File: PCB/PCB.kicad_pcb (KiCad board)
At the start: 2 copper layers, 17 parts, among them U1 ESP32-WROOM-32E-N8R2

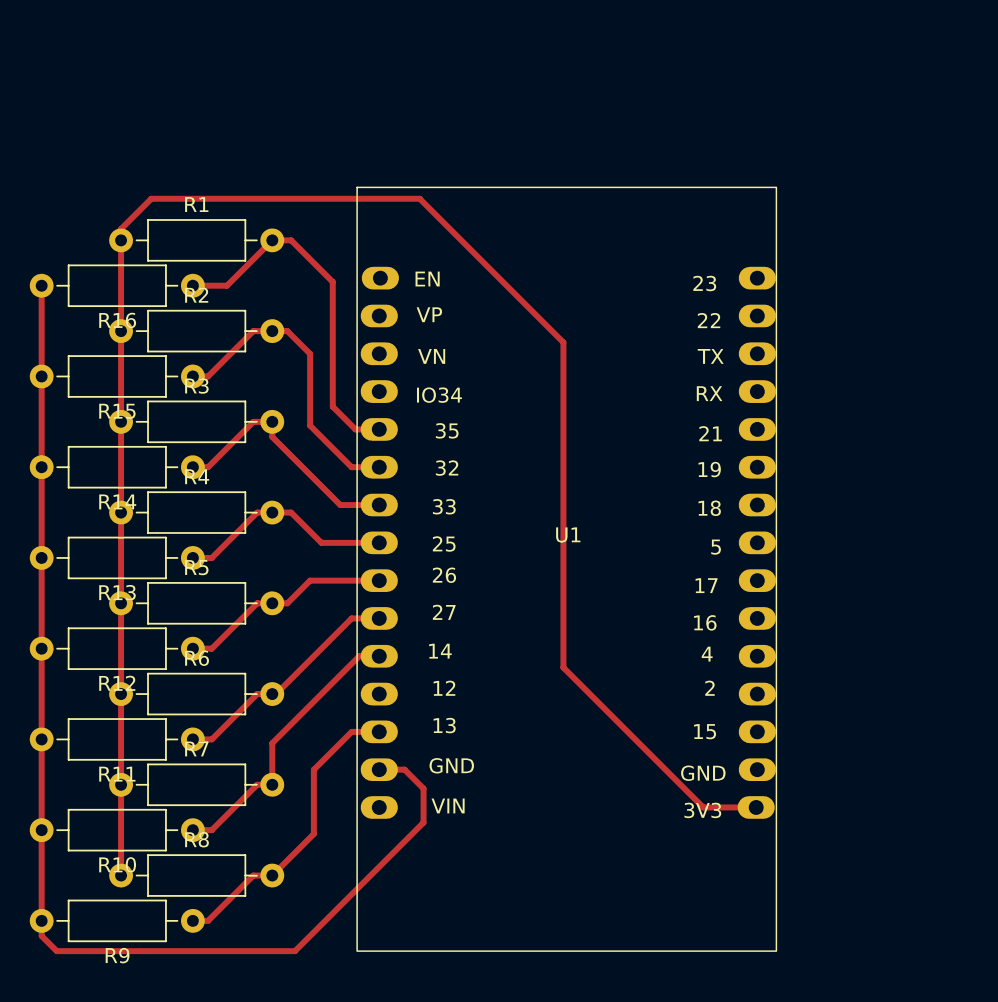
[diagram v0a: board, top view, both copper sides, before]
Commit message: updates
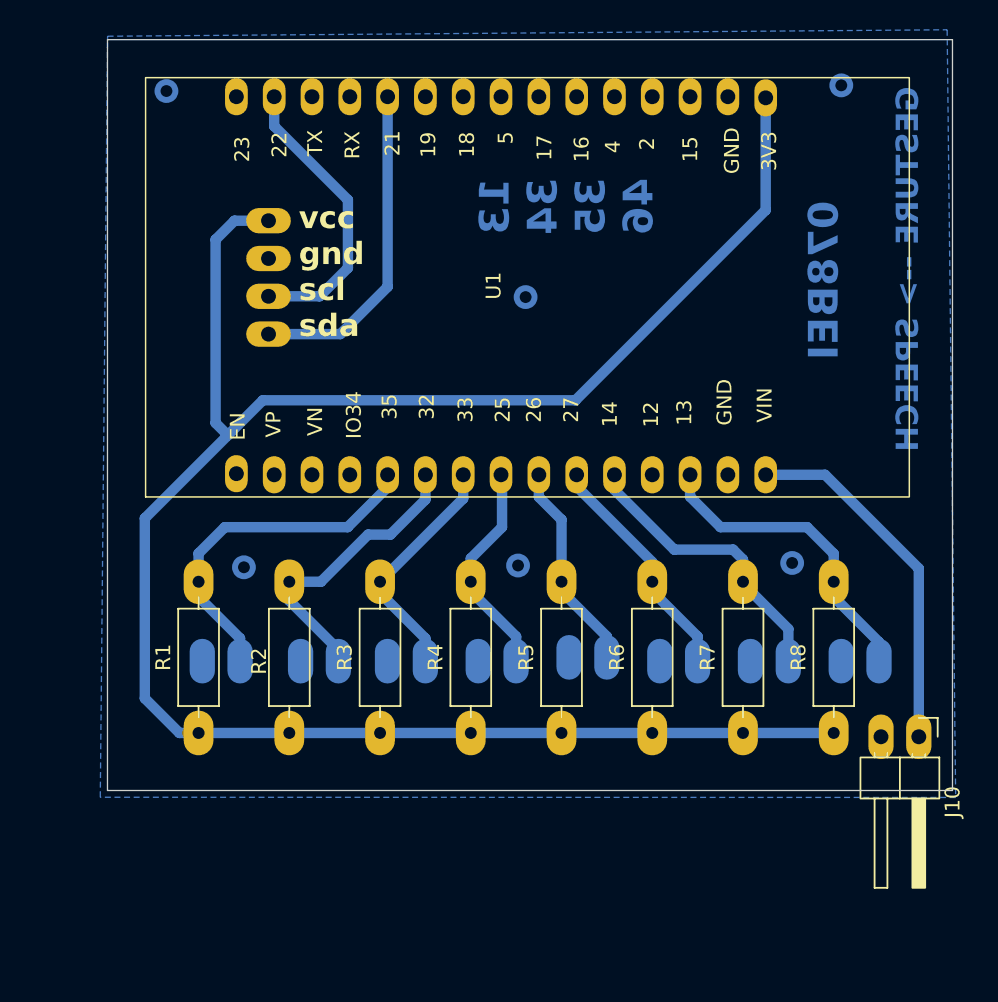
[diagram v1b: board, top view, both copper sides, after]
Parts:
- removed R10, R11, R12, R13, R14, R15, R16, R9: R, Resistor_THT:R_Axial_DIN0207_L6.3mm_D2.5mm_P10.16mm_Horizontal
- added J1: Conn_01x02_Pin, symbols_footprint:PinHeader_1x02_P2.54mm_Vertical smd custom, F.Cu at (170.6, 98.9)
- added J10: Conn_01x02_Pin, Connector_PinHeader_2.54mm:PinHeader_1x02_P2.54mm_Horizontal, F.Cu at (175.8, 104.0)
- added J2: Conn_01x02_Pin, symbols_footprint:PinHeader_1x02_P2.54mm_Vertical smd custom, F.Cu at (164.5, 98.9)
- added J3: Conn_01x02_Pin, symbols_footprint:PinHeader_1x02_P2.54mm_Vertical smd custom, F.Cu at (158.4, 98.9)
- added J4: Conn_01x02_Pin, symbols_footprint:PinHeader_1x02_P2.54mm_Vertical smd custom, F.Cu at (152.3, 98.6)
- added J5: Conn_01x02_Pin, symbols_footprint:PinHeader_1x02_P2.54mm_Vertical smd custom, F.Cu at (146.2, 98.9)
- added J6: Conn_01x02_Pin, symbols_footprint:PinHeader_1x02_P2.54mm_Vertical smd custom, F.Cu at (140.1, 98.9)
- added J7: Conn_01x02_Pin, symbols_footprint:PinHeader_1x02_P2.54mm_Vertical smd custom, F.Cu at (134.2, 98.9)
- added J8: Conn_01x02_Pin, symbols_footprint:PinHeader_1x02_P2.54mm_Vertical smd custom, F.Cu at (127.6, 98.9)
- added J9: Conn_01x04_Pin, Connector_PinHeader_2.54mm:PinHeader_1x04_P2.54mm_Vertical, F.Cu at (132.1, 69.3)
- moved R8 48.8 mm to (170.1, 103.7), turned to 90 degrees
- moved R7 41.9 mm to (164.0, 103.7), turned to 90 degrees
- moved R6 35.8 mm to (157.9, 103.7), turned to 90 degrees
- moved R1 33.5 mm to (127.4, 103.7), turned to 90 degrees
- moved R5 30.8 mm to (151.8, 103.7), turned to 90 degrees
- moved R2 29.3 mm to (133.5, 103.7), turned to 90 degrees
- moved R4 27.8 mm to (145.7, 103.7), turned to 90 degrees
- moved R3 27.2 mm to (139.6, 103.7), turned to 90 degrees
- moved U1 17.9 mm to (147.7, 73.7), turned to 90 degrees
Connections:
- U1 pad 15: unconnected-(U1-VIN-Pad15) -> /VIN
- U1 pad 26: unconnected-(U1-IO21-Pad26) -> /SDA
- U1 pad 29: unconnected-(U1-IO22-Pad29) -> /SCL
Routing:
- net /GND: track 79.1 -> 0.00 mm
- net /VIN: track 0.00 -> 24.2 mm
- net /SDA: track 0.00 -> 22.1 mm
- net /SCL: track 0.00 -> 19.7 mm
- net /3V3: track 117.0 -> 135.9 mm
- net /IO25: track 14.6 -> 17.0 mm
- net /IO13: track 20.3 -> 22.5 mm
- net /IO26: track 14.4 -> 16.4 mm
- net /IO14: track 19.0 -> 20.7 mm
- net /IO32: track 20.4 -> 22.0 mm
- net /IO27: track 15.9 -> 17.2 mm
- net /IO35: track 24.0 -> 25.0 mm
- net /IO33: track 16.7 -> 17.4 mm
- added copper zone on B.Cu, net /GND
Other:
- board outline added: 56.8 x 50.4 mm
- board text added: "078BEI"
- board text added: "13 34 35 46"
- board text added: "GESTURE --> SPEECH"
- board text added: "vcc gnd scl sda"
